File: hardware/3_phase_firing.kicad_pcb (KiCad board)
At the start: 2 copper layers, 142.5 x 77.5 mm, 61 parts, among them J1 IN1, J2 IN2, J3 OUT, Q1 MMBT3904, Q2 MMBT3904, Q3 MMBT3904, Q4 MMBT3904, Q5 MMBT3904, Q6 MMBT3904, U1 LM339, U10 4N35, U11 4N35, U12 4N35, U2 L7812, U3 4N35, U4 4N35, U5 4N35, U6 YAAJ_WeAct_BlackPill_Part_Like, U7 4N35, U8 4N35, U9 4N35

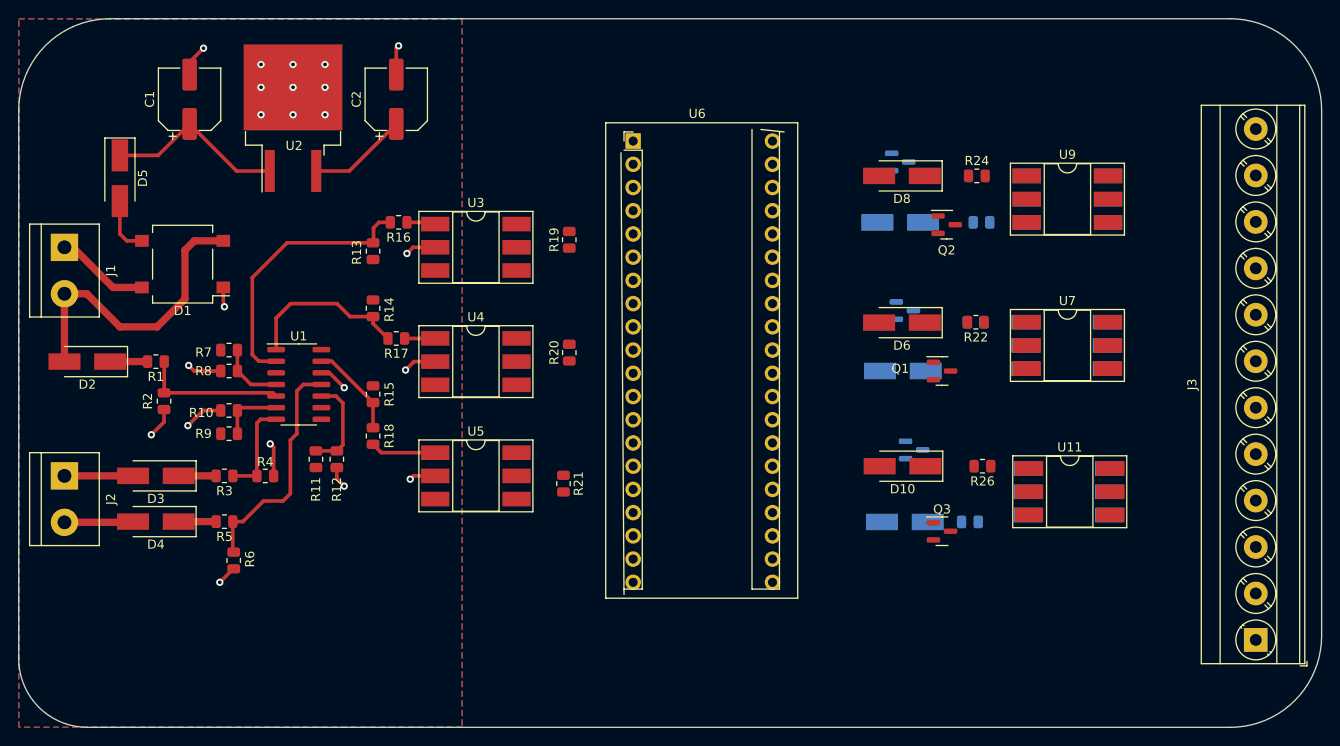
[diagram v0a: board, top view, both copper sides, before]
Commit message: fixing kicad_pcb files
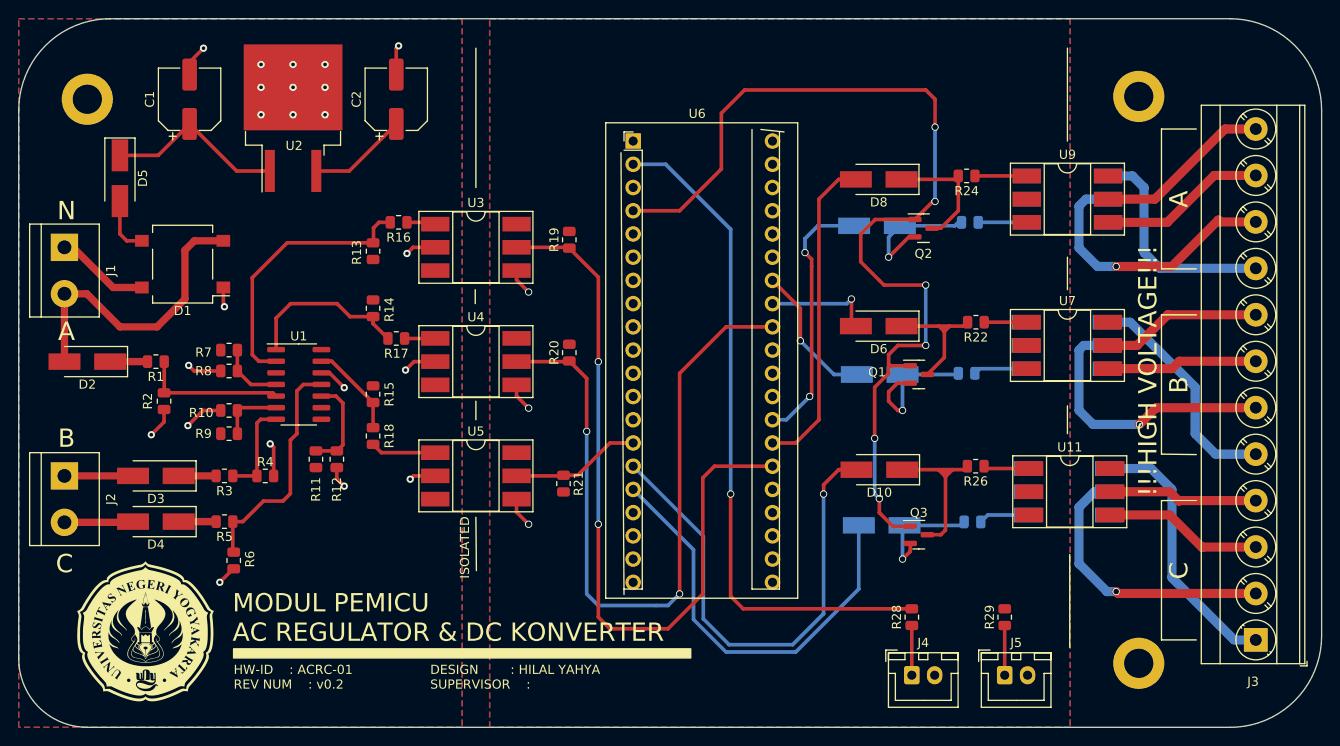
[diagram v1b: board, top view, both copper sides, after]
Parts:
- removed Q4, Q5, Q6: MMBT3904, Package_TO_SOT_SMD:SOT-23
- added G***: LOGO, logo_uny:logo_uny_15mm, F.Cu at (86.4, 109.5)
- added J4: USB_LED, Connector_JST:JST_XH_B2B-XH-A_1x02_P2.50mm_Vertical, F.Cu at (170.2, 114.3)
- added J5: POWER, Connector_JST:JST_XH_B2B-XH-A_1x02_P2.50mm_Vertical, F.Cu at (180.3, 114.3)
- added R28: 220, Resistor_SMD:R_0805_2012Metric, F.Cu at (170.2, 108.0)
- added R29: 220, Resistor_SMD:R_0805_2012Metric, F.Cu at (180.3, 108.0)
- added REF**: MountingHole_3.2mm_M3_DIN965_Pad, MountingHole:MountingHole_3.2mm_M3_DIN965_Pad, F.Cu at (195.0, 113.0)
- added REF**: MountingHole_3.2mm_M3_DIN965_Pad, MountingHole:MountingHole_3.2mm_M3_DIN965_Pad, F.Cu at (80.0, 51.3)
- added REF**: MountingHole_3.2mm_M3_DIN965_Pad, MountingHole:MountingHole_3.2mm_M3_DIN965_Pad, F.Cu at (195.0, 51.0)
- moved R23 5.67 mm to (176.2, 81.3), turned to 180 degrees
- moved D11 2.57 mm to (166.9, 97.9)
- moved D6 2.57 mm to (166.6, 76.1)
- moved D7 2.57 mm to (166.7, 81.4)
- moved D8 2.57 mm to (166.6, 60.1)
- moved Q2 2.57 mm to (171.4, 65.4)
- moved D10 2.57 mm to (166.6, 91.8)
- moved D9 2.57 mm to (166.4, 65.2)
- moved Q1 2.57 mm to (170.9, 81.4)
- moved Q3 2.57 mm to (170.9, 98.9)
- moved R25 1.27 mm to (176.5, 64.8), turned to 180 degrees
- moved R24 1.12 mm to (176.2, 59.7), turned to 180 degrees
- moved R26 0.74 mm to (177.2, 91.4)
- moved R27 0.28 mm to (176.8, 97.5)
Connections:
- U6 pad 14: unconnected-(U6-Pad14) -> ZCD_C
- U6 pad 15: unconnected-(U6-Pad15) -> GATE_C1
- U6 pad 16: unconnected-(U6-Pad16) -> GATE_C2
- U6 pad 2: unconnected-(U6-Pad2) -> LED_USB
- U6 pad 32: unconnected-(U6-Pad32) -> ZCD_B
- U6 pad 33: unconnected-(U6-Pad33) -> GATE_B1
- U6 pad 34: unconnected-(U6-Pad34) -> GATE_B2
- U6 pad 4: unconnected-(U6-Pad4) -> TRIAC_MODE
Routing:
- net TRIAC_MODE: track 0.00 -> 110.2 mm, vias 0 -> 6
- net ZCD_A: track 0.00 -> 81.9 mm, vias 0 -> 2
- net ZCD_B: track 0.00 -> 79.7 mm, vias 0 -> 2
- net LED_USB: track 0.00 -> 74.1 mm, vias 0 -> 1
- net GATE_C1: track 0.00 -> 54.0 mm, vias 0 -> 1
- net GATE_C2: track 0.00 -> 46.3 mm
- net GATE_A1: track 0.00 -> 35.2 mm
- net OUTC2_C: track 0.00 -> 30.9 mm, vias 0 -> 1
- net OUTB2_C: track 0.00 -> 30.6 mm, vias 0 -> 1
- net OUTA2_C: track 0.00 -> 30.4 mm, vias 0 -> 1
- net OUTC2_E: track 0.00 -> 29.4 mm
- net GATE_A2: track 0.00 -> 28.7 mm, vias 0 -> 2
- net OUTB2_E: track 0.00 -> 25.2 mm
- net OUTA2_E: track 0.00 -> 24.5 mm
- net Net-(D10-Pad1): track 0.00 -> 19.8 mm
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- added copper zone on F.Cu, net +3.3V
- added copper zone on B.Cu, net GND
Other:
- board text added: "!!!HIGH VOLTAGE!!!"
- board text added: "A"
- board text added: "B"
- board text added: "C"
- board text added: "DESIGN : HILAL YAHYA SUPERVISOR :"
- board text added: "HW-ID : ACRC-01 REV NUM : v0.2"
- board text added: "ISOLATED"
- board text added: "MODUL PEMICU AC REGULATOR & DC KONVERTER"
- board text added: "N"

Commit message: Revert "tracing path of the pcb"
This reverts commit a1f78cd755137d86b9aab8dfdd90e54233a75f74.
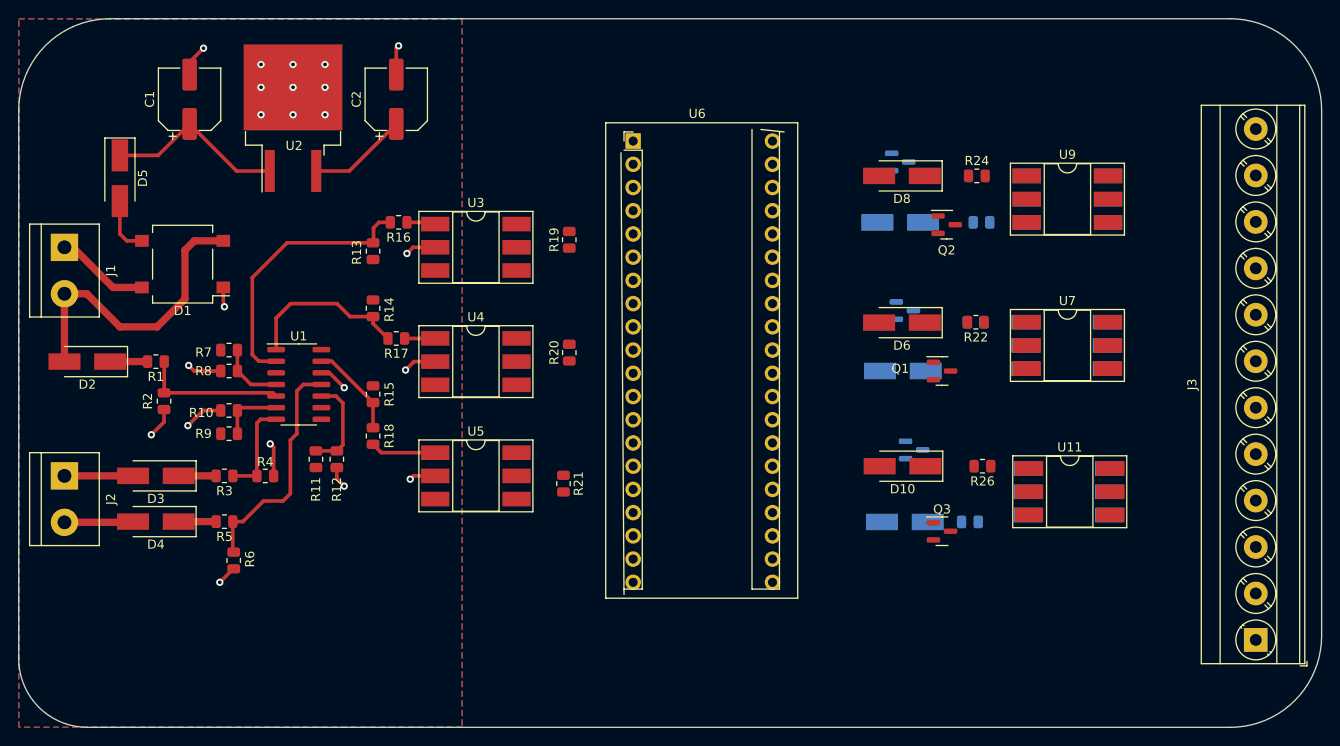
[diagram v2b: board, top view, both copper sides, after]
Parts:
- removed G***: LOGO, logo_uny:logo_uny_15mm
- removed J4: USB_LED, Connector_JST:JST_XH_B2B-XH-A_1x02_P2.50mm_Vertical
- removed J5: POWER, Connector_JST:JST_XH_B2B-XH-A_1x02_P2.50mm_Vertical
- removed R28, R29: 220, Resistor_SMD:R_0805_2012Metric
- removed REF** (x3): MountingHole_3.2mm_M3_DIN965_Pad, MountingHole:MountingHole_3.2mm_M3_DIN965_Pad
- added Q4: MMBT3904, Package_TO_SOT_SMD:SOT-23, B.Cu at (169.4, 74.4)
- added Q5: MMBT3904, Package_TO_SOT_SMD:SOT-23, B.Cu at (168.9, 58.2)
- added Q6: MMBT3904, Package_TO_SOT_SMD:SOT-23, B.Cu at (170.4, 89.7)
- moved R23 5.67 mm to (177.1, 75.7), turned to 0 degrees
- moved D11 2.57 mm to (169.4, 97.5)
- moved D6 2.57 mm to (169.1, 75.7)
- moved D7 2.57 mm to (169.2, 81.0)
- moved D8 2.57 mm to (169.1, 59.7)
- moved Q2 2.57 mm to (174.0, 65.0)
- moved D10 2.57 mm to (169.2, 91.4)
- moved D9 2.57 mm to (168.9, 64.8)
- moved Q1 2.57 mm to (173.5, 81.0)
- moved Q3 2.57 mm to (173.5, 98.6)
- moved R25 1.27 mm to (177.8, 64.8), turned to 0 degrees
- moved R24 1.12 mm to (177.3, 59.7), turned to 0 degrees
- moved R26 0.74 mm to (177.9, 91.4)
- moved R27 0.28 mm to (176.5, 97.5)
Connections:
- U6 pad 14: ZCD_C -> unconnected-(U6-Pad14)
- U6 pad 15: GATE_C1 -> unconnected-(U6-Pad15)
- U6 pad 16: GATE_C2 -> unconnected-(U6-Pad16)
- U6 pad 2: LED_USB -> unconnected-(U6-Pad2)
- U6 pad 32: ZCD_B -> unconnected-(U6-Pad32)
- U6 pad 33: GATE_B1 -> unconnected-(U6-Pad33)
- U6 pad 34: GATE_B2 -> unconnected-(U6-Pad34)
- U6 pad 4: TRIAC_MODE -> unconnected-(U6-Pad4)
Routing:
- net TRIAC_MODE: track 110.2 -> 0.00 mm, vias 6 -> 0
- net ZCD_A: track 81.9 -> 0.00 mm, vias 2 -> 0
- net ZCD_B: track 79.7 -> 0.00 mm, vias 2 -> 0
- net LED_USB: track 74.1 -> 0.00 mm, vias 1 -> 0
- net GATE_C1: track 54.0 -> 0.00 mm, vias 1 -> 0
- net GATE_C2: track 46.3 -> 0.00 mm
- net GATE_A1: track 35.2 -> 0.00 mm
- net OUTC2_C: track 30.9 -> 0.00 mm, vias 1 -> 0
- net OUTB2_C: track 30.6 -> 0.00 mm, vias 1 -> 0
- net OUTA2_C: track 30.4 -> 0.00 mm, vias 1 -> 0
- net OUTC2_E: track 29.4 -> 0.00 mm
- net GATE_A2: track 28.7 -> 0.00 mm, vias 2 -> 0
- net OUTB2_E: track 25.2 -> 0.00 mm
- net OUTA2_E: track 24.5 -> 0.00 mm
- net Net-(D10-Pad1): track 19.8 -> 0.00 mm
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- removed copper zone on F.Cu, net +3.3V
- removed copper zone on B.Cu, net GND
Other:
- board text removed: "!!!HIGH VOLTAGE!!!"
- board text removed: "A"
- board text removed: "B"
- board text removed: "C"
- board text removed: "DESIGN : HILAL YAHYA SUPERVISOR :"
- board text removed: "HW-ID : ACRC-01 REV NUM : v0.2"
- board text removed: "ISOLATED"
- board text removed: "MODUL PEMICU AC REGULATOR & DC KONVERTER"
- board text removed: "N"
